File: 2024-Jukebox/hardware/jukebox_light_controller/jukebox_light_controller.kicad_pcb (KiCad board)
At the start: 2 copper layers, 100 x 100 mm, 179 parts, among them J1 HEAD_LEDS, J10 BUTTON_3, J11 BUTTON_4, J12 BUTTON_5, J13 BUTTON_6, J14 BUTTON_7, J15 VOLUME, J16 DISPLAY_1, J17 DISPLAY_2, J2 MOUTH_LEDS, J3 76829-0004, J4 Conn_01x03, J5 ROTARY_SWITCH, J6 BUTTON_1, J7 USB_C_Receptacle_USB2.0, J8 BUTTON_2, J9 RJ45_Wuerth_7499010121A, Q1 2N7002, Q2 2N7002, Q3 BSS138, Q4 BSS138, Q5 BSS138, Q6 BSS138, Q7 BSS138, Q8 BSS138, Q9 BSS138, SW1 SW_DIP_x03, SW2 SW_Push, SW3 SW_Push, U12 W25Q128JVS, U4 AMS1117-3.3, U5 RP2040, U6 W5500, Y1 12MHz, Y2 25MHz

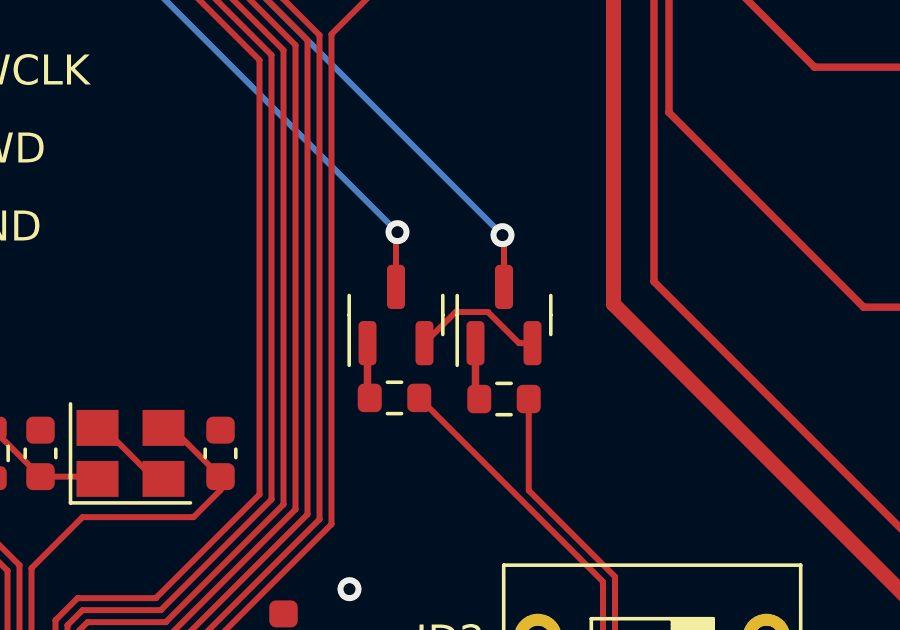
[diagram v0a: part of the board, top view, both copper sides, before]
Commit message: Updated schematic
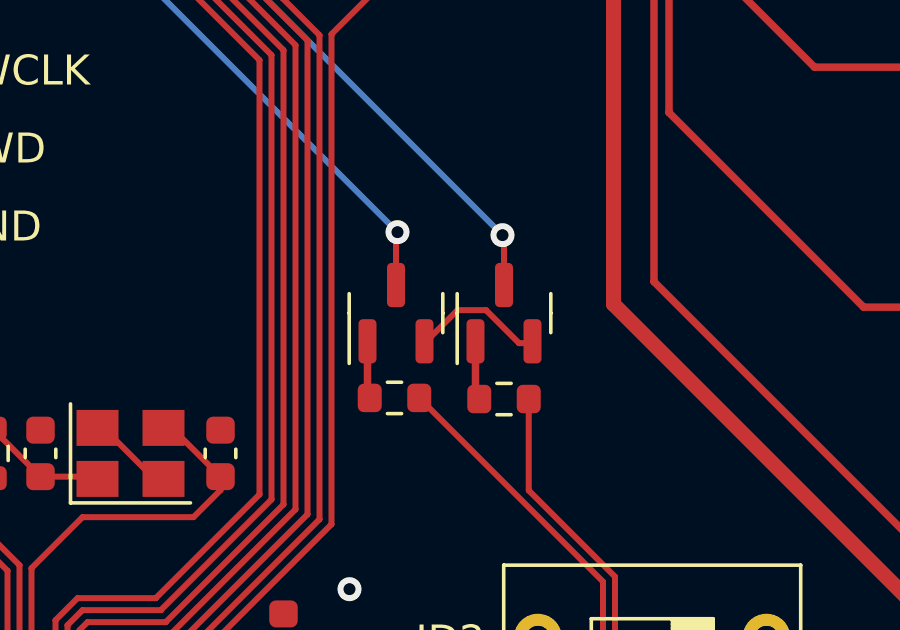
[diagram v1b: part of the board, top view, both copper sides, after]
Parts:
- removed Q2: 2N7002, Package_TO_SOT_SMD:SOT-23
- added Q10: MMBT2222, Package_TO_SOT_SMD:SOT-23, F.Cu at (60.6, 59.1)
- Q1: value 2N7002 -> MMBT2222
- R79, R80: value 100 -> 470
- moved Q1 0.06 mm to (64.2, 59.1)
